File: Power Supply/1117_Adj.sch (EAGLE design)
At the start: 4 parts

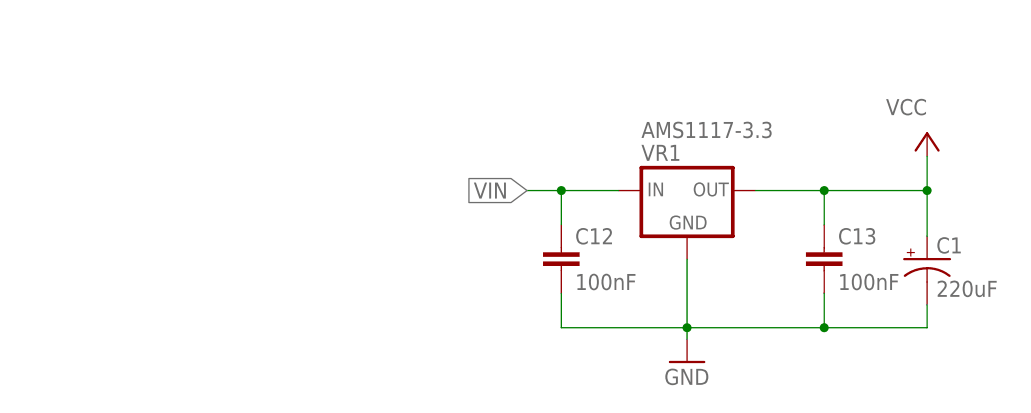
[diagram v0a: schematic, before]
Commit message: few ckt updated
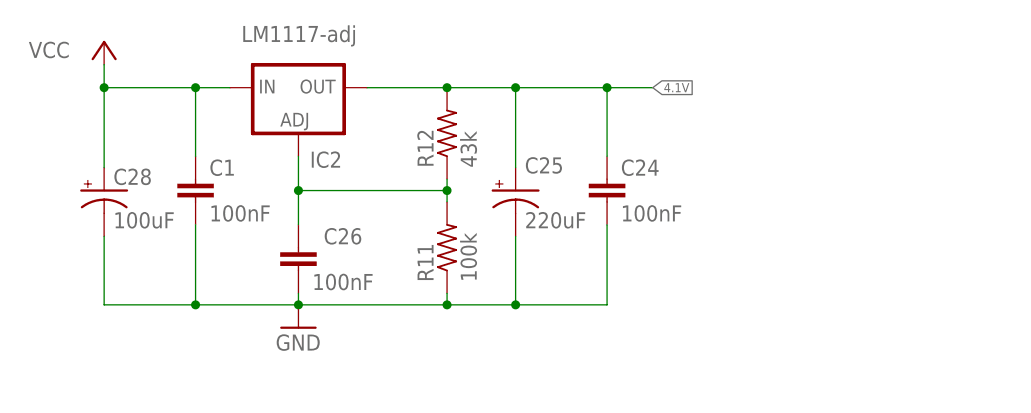
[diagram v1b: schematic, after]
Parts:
- removed C12, C13: 100nF, rcl:C-EU050-024X044
- removed VR1: AMS1117-3.3, PatternAgents-OnSemi:NCP1117ST50T3G
- added C24, C26: 100nF, rcl:C-EU050-024X044
- added C25: 220uF, rcl:CPOL-USE2.5-6
- added C28: 100uF, rcl:CPOL-USE2.5-6
- added IC2: LM1117-adj, v-reg:LD117AS25TR
- added R11: 100k, resistor:R-US_0204/7
- added R12: 43k, resistor:R-US_0204/7
- C1: value 220uF -> 100nF; device rcl:CPOL-USTT2D6 -> rcl:C-EU050-024X044
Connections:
- removed net VIN: C12.1, VR1.IN
- new net 4.1V: C24.1, C25.+, IC2.OUT, R12.2
- new net N$5: C26.1, IC2.ADJ, R11.2, R12.1
- net GND: now also C1.2, C24.2, C25.-, C26.2, C28.-, R11.1; no longer C1.-, C12.2, C13.2, VR1.GND
- net VCC: now also C1.1, C28.+, IC2.IN; no longer C1.+, C13.1, VR1.OUT
